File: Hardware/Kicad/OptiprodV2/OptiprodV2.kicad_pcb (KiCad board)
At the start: 2 copper layers, 12 parts, among them U1 MCP6002-xMC, U2 BME280

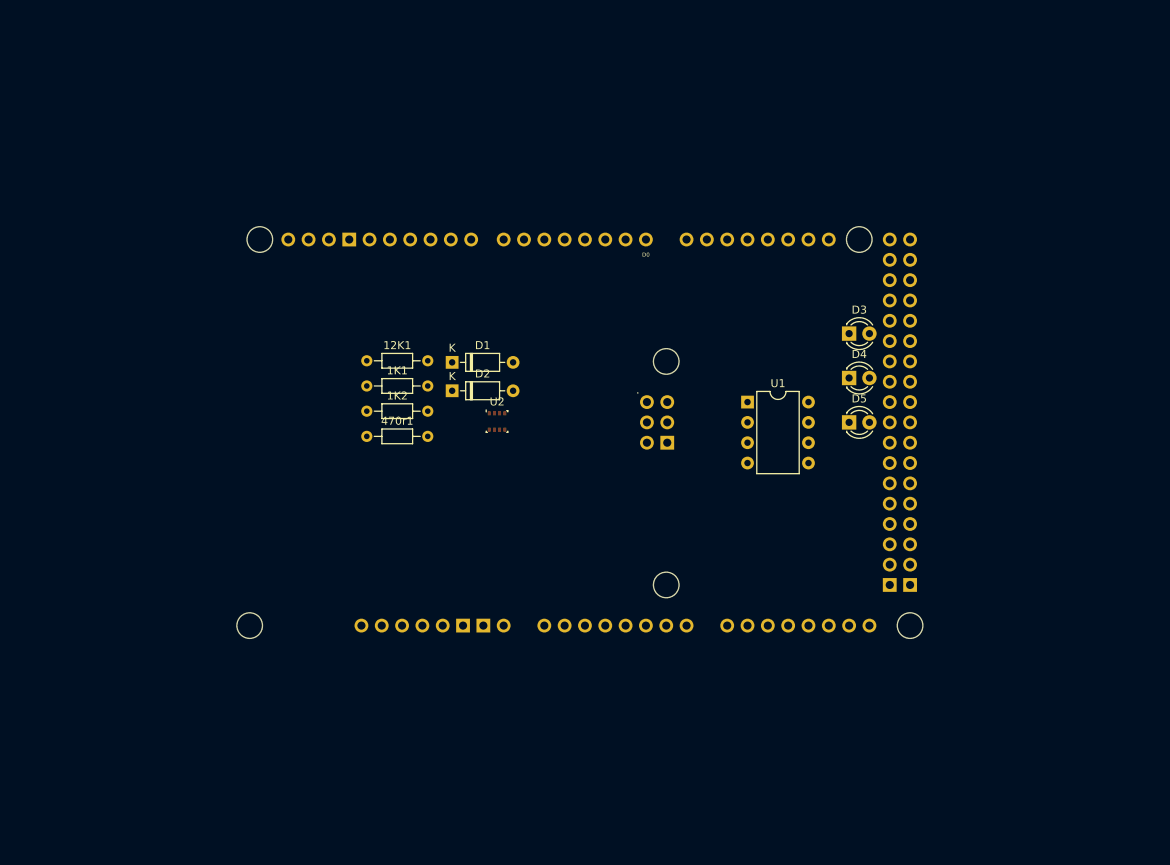
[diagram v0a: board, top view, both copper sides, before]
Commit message: commit2.2.1
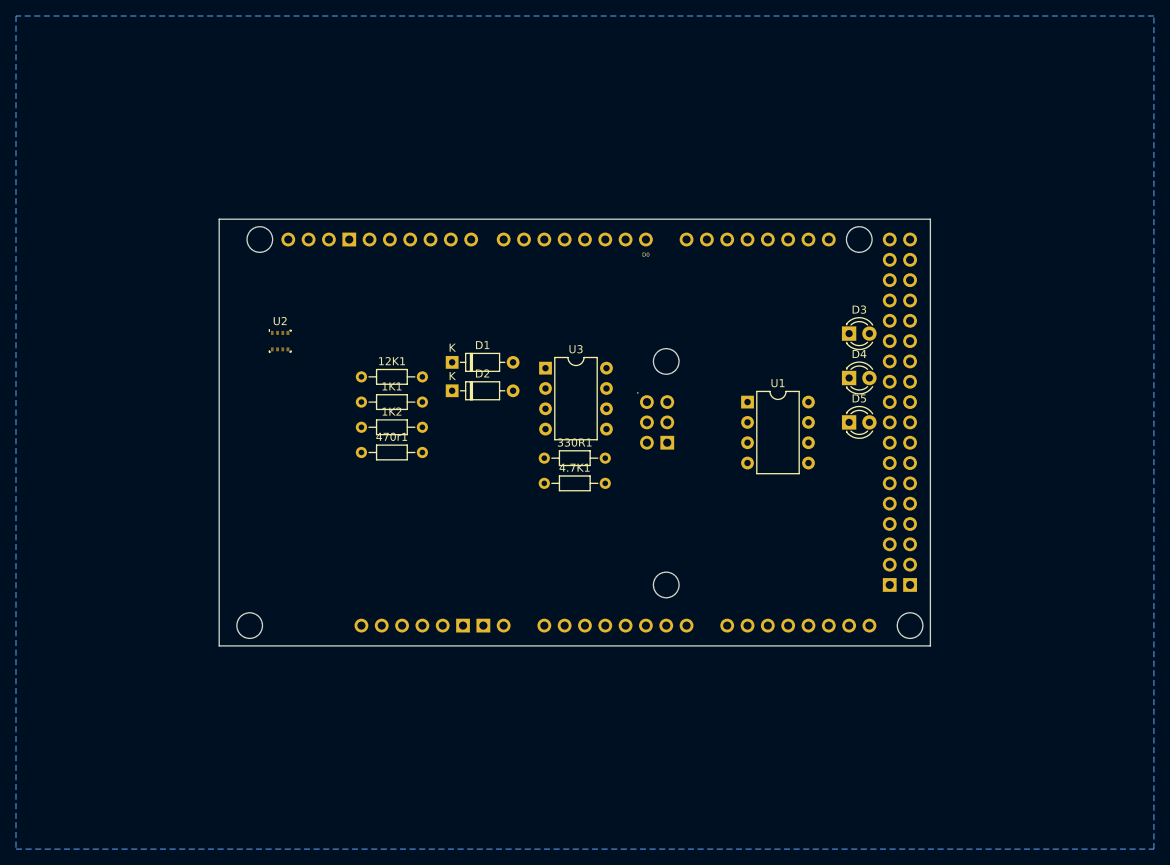
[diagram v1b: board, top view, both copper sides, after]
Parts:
- added 330R1: R, Resistor_THT:R_Axial_DIN0204_L3.6mm_D1.6mm_P7.62mm_Horizontal, F.Cu at (144.8, 83.2)
- added 4.7K1: R, Resistor_THT:R_Axial_DIN0204_L3.6mm_D1.6mm_P7.62mm_Horizontal, F.Cu at (144.8, 86.4)
- added U3: TL082, Package_DIP:DIP-8_W7.62mm, F.Cu at (144.9, 72.0)
- moved U2 28.9 mm to (111.8, 68.6)
- moved 1K1 2.12 mm to (121.9, 76.2)
- moved 12K1 2.12 mm to (121.9, 73.0)
- moved 1K2 2.12 mm to (121.9, 79.3)
- moved 470r1 2.12 mm to (121.9, 82.5)
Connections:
- A2 pad A0: unconnected-(A2-PadA0) -> Net-(U3B--)
- U1 pad 3: Net-(D2-K) -> Net-(DZ3-K)
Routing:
- added copper zone on B.Cu, net GND
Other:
- board outline added: 88.9 x 53.3 mm
